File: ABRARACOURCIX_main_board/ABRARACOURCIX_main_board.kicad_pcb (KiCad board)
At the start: 2 copper layers, 140 x 140 mm, 78 parts, among them J1 Conn_01x05_Socket, J10 XT60PW-M, J11 Conn_01x02_Pin, J12 Conn_01x02_Pin, J2 Conn_01x06_Socket, J3 Conn_01x03_Socket, J4 Conn_01x03_Socket, J5 Conn_01x03_Socket, J6 Conn_01x03_Socket, J7 Conn_01x03_Socket, J8 XT60PW-M, J9 XT60PW-F, Q2 DSS20200L-7-PNP, Q3 IKD15N60R, Q4 NPN-DSS20201L-7, Q5 NTR4101PT1G, U1 STM32F429VITx, U2 BNO055, U3 Current_sens_ACS712ELCTR-20A-T, U4 AZ1117CH-3.3TRG1, U5 LMC6482AIMX/NOPB, U6 LMC6482AIMX/NOPB, Y1 ABS07-32.768KHZ-T

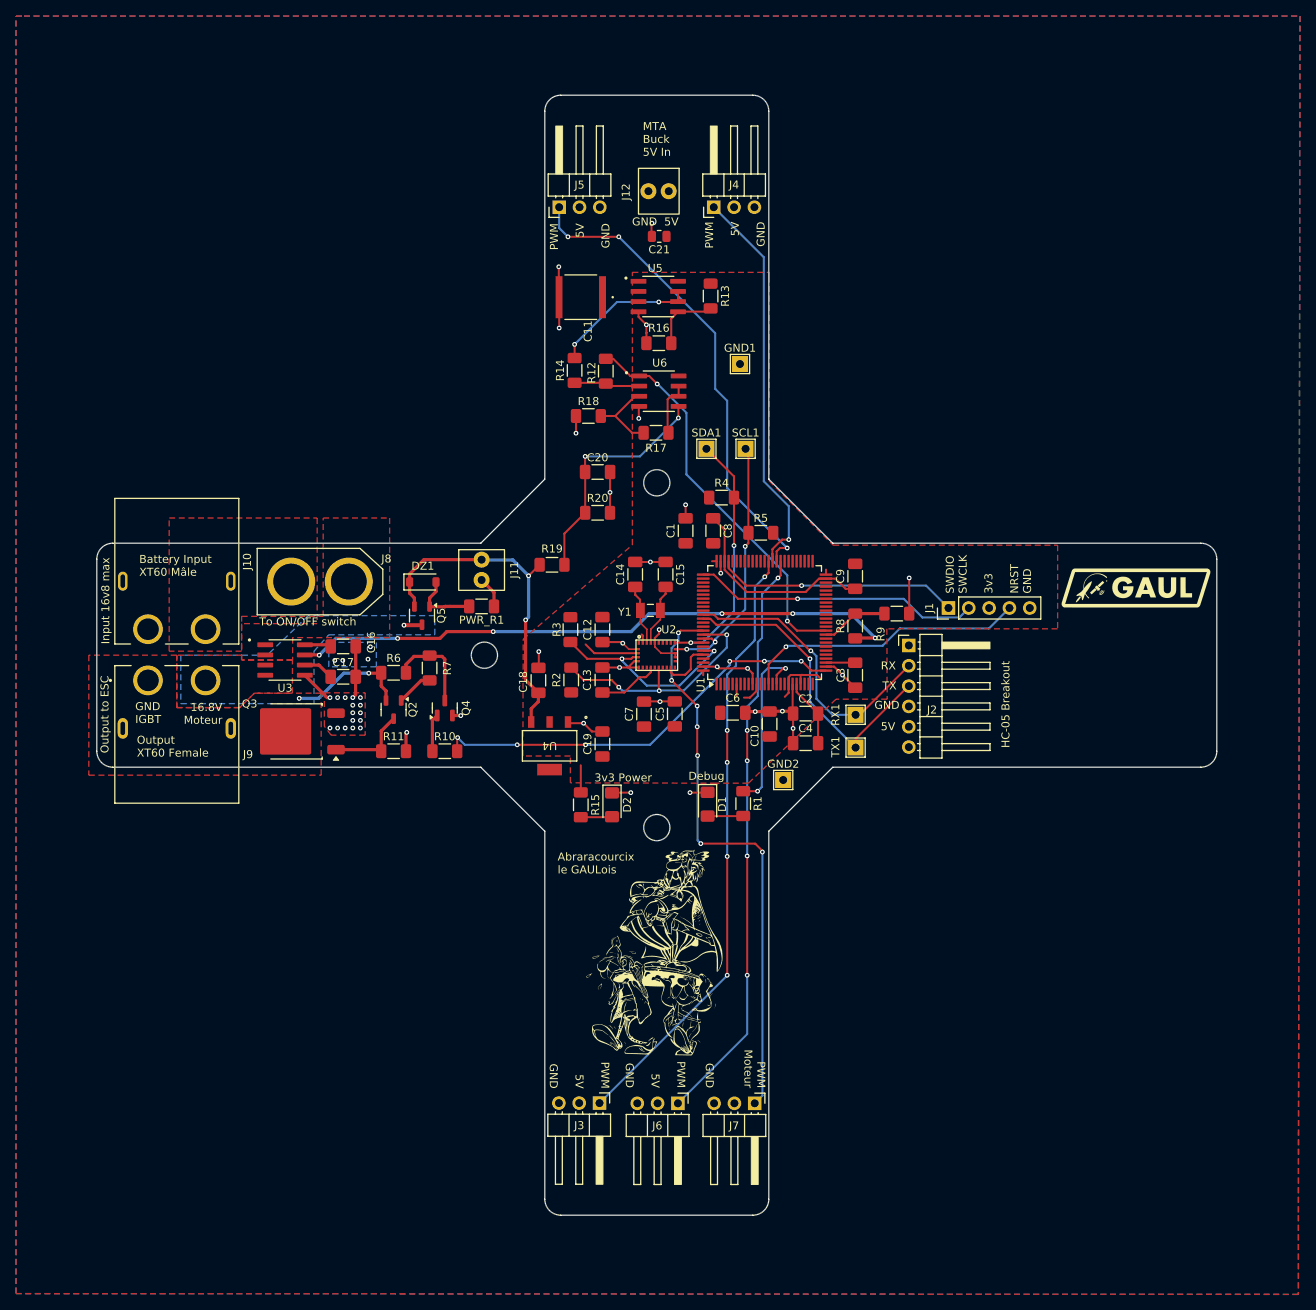
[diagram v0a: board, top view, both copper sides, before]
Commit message: Circuit+début PCB
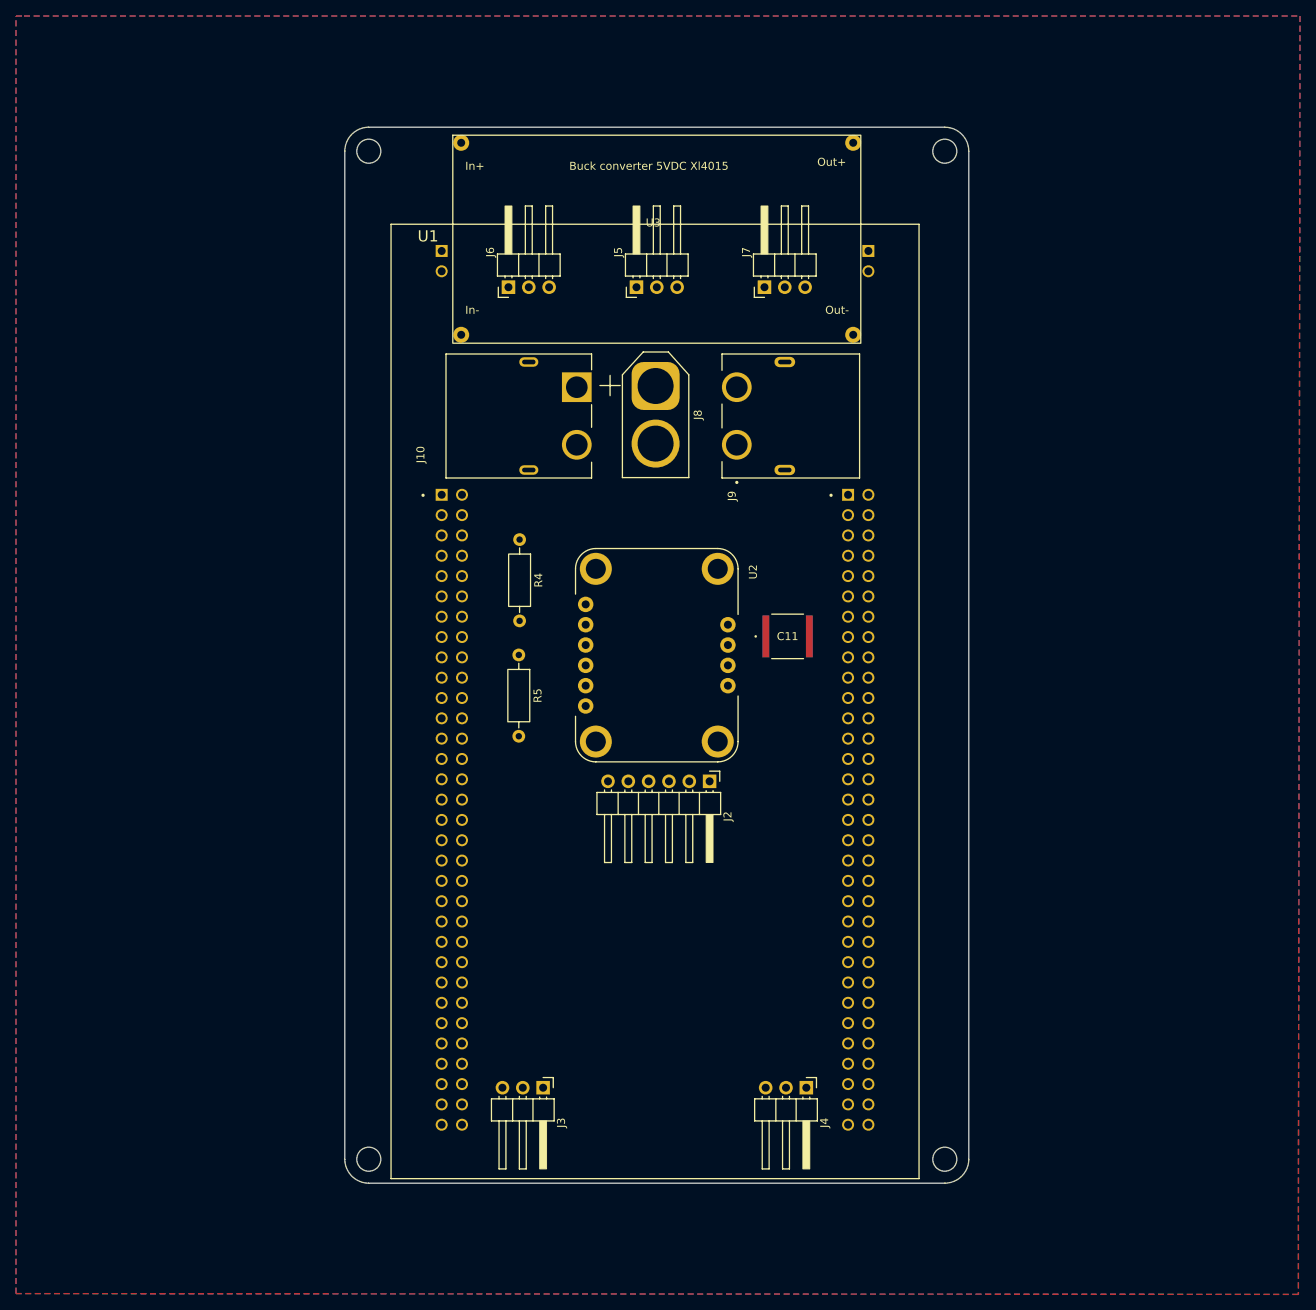
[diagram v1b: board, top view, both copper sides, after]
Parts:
- removed Abraracourcix_moyen: LOGO, Librairie_footprint:Abraracourcix_moyen
- removed C1, C2, C3, C5, C6: 100n, Capacitor_SMD:C_1206_3216Metric_Pad1.33x1.80mm_HandSolder
- removed C10, C20, C4: 1u, Capacitor_SMD:C_1206_3216Metric_Pad1.33x1.80mm_HandSolder
- removed C12: 100nF, Capacitor_SMD:C_1206_3216Metric_Pad1.33x1.80mm_HandSolder
- removed C13: 1uF, Capacitor_SMD:C_1206_3216Metric_Pad1.33x1.80mm_HandSolder
- removed C14, C15: 22pF, Capacitor_SMD:C_1206_3216Metric_Pad1.33x1.80mm_HandSolder
- removed C16: 0.1u, Capacitor_SMD:C_1206_3216Metric_Pad1.33x1.80mm_HandSolder
- removed C17: 1n, Capacitor_SMD:C_1206_3216Metric_Pad1.33x1.80mm_HandSolder
- removed C18: 10u, Capacitor_SMD:C_1206_3216Metric_Pad1.33x1.80mm_HandSolder
- removed C19: 22u, Capacitor_SMD:C_1206_3216Metric_Pad1.33x1.80mm_HandSolder
- removed C21: 22u, Resistor_SMD:R_0805_2012Metric
- removed C7: 4.7u, Capacitor_SMD:C_1206_3216Metric_Pad1.33x1.80mm_HandSolder
- removed C8, C9: 2.2u, Capacitor_SMD:C_1206_3216Metric_Pad1.33x1.80mm_HandSolder
- removed D1, D2: 599-0410-127F, Diode_SMD:D_1206_3216Metric_Pad1.42x1.75mm_HandSolder
- removed DZ1: SZMMSZ4679T1G, Diode_SMD:D_SOD-123
- removed G***1, G***2, G***3: LOGO, LOGO
- removed GND1, GND2, RX1, SCL1, SDA1, TX1: TestPoint, TestPoint:TestPoint_THTPad_2.0x2.0mm_Drill1.0mm
- removed J1: Conn_01x05_Socket, Connector_PinHeader_2.54mm:PinHeader_1x05_P2.54mm_Vertical
- removed J11, J12: Conn_01x02_Pin, Librairie_footprint:MTA_100_2pos
- removed PWR_R1: 100k, Resistor_SMD:R_1206_3216Metric_Pad1.30x1.75mm_HandSolder
- removed Q2: DSS20200L-7-PNP, Package_TO_SOT_SMD:SOT-23-3
- removed Q3: IKD15N60R, Package_TO_SOT_SMD:TO-252-2
- removed Q4: NPN-DSS20201L-7, Package_TO_SOT_SMD:SOT-23
- removed Q5: NTR4101PT1G, Package_TO_SOT_SMD:SOT-23-3
- removed R1, R15: 40, Resistor_SMD:R_1206_3216Metric_Pad1.30x1.75mm_HandSolder
- removed R10, R7: 1k5, Resistor_SMD:R_1206_3216Metric_Pad1.30x1.75mm_HandSolder
- removed R11, R13, R14, R17, R20, R6, R8: 10k, Resistor_SMD:R_1206_3216Metric_Pad1.30x1.75mm_HandSolder
- removed R12, R16, R18: 30k, Resistor_SMD:R_1206_3216Metric_Pad1.30x1.75mm_HandSolder
- removed R19: 40k, Resistor_SMD:R_1206_3216Metric_Pad1.30x1.75mm_HandSolder
- removed R2, R3: 10K, Resistor_SMD:R_1206_3216Metric_Pad1.30x1.75mm_HandSolder
- removed R9: 20k, Resistor_SMD:R_1206_3216Metric_Pad1.30x1.75mm_HandSolder
- removed U4: AZ1117CH-3.3TRG1, Librairie_footprint:AZ1117CH_3_3TRG1-L
- removed U5, U6: LMC6482AIMX/NOPB, Librairie_footprint:SOIC127P599X175-8N
- removed Y1: ABS07-32.768KHZ-T, Librairie_footprint:XTAL_ABS07-32.768KHZ-T
- added ?: , , F.Cu at (-36.0, 63.0)
- added ?: , , F.Cu at (-36.0, -62.1)
- added ?: , , F.Cu at (35.0, -63.8)
- added ?: , , F.Cu at (35.6, 63.0)
- R4, R5: footprint Resistor_SMD:R_1206_3216Metric_Pad1.30x1.75mm_HandSolder -> Resistor_THT:R_Axial_DIN0207_L6.3mm_D2.5mm_P10.16mm_Horizontal
- U1: value STM32F429VITx -> STM32F429I-DISC1; footprint Package_QFP:LQFP-100_14x14mm_P0.5mm -> Librairie_footprint:MODULE_STM32F429I-DISC1
- U2: value BNO055 -> BNO055_breakout; footprint Librairie_footprint:BNO055_LGA28R50P4X10_380X520X100 -> Librairie_footprint:MODULE_2472
- U3: value Current_sens_ACS712ELCTR-20A-T -> ~; footprint Librairie_footprint:Current_sens_SOIC127P600X175-8N -> Librairie_footprint:Buck_breakout_Xl4015
- moved J4 110.7 mm to (18.7, 54.1), turned to -90 degrees
- moved J6 103.7 mm to (-16.0, -46.0), turned to 90 degrees
- moved J7 102.1 mm to (16.0, -46.0), turned to 90 degrees
- moved J9 79.0 mm to (10.0, -33.5), turned to 90 degrees
- moved U3 70.2 mm to (0.00, -52.0)
- moved J10 55.6 mm to (-10.0, -33.5), turned to 90 degrees
- moved C11 49.7 mm to (16.4, -2.35), turned to 0 degrees
- moved J8 45.5 mm to (-0.15, -33.6), turned to -90 degrees
- moved R5 33.9 mm to (-17.2, -0.03), turned to -90 degrees
- moved J2 30.1 mm to (6.60, 15.8), turned to -90 degrees
- moved R4 25.8 mm to (-17.1, -14.4), turned to -90 degrees
- moved U1 16.9 mm to (-0.22, 5.78), turned to 0 degrees
- moved J5 15.8 mm to (0.00, -46.0)
- moved J3 7.31 mm to (-14.2, 54.1)
- turned U2 to -90 degrees
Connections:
- J2 pad 2: HC_RX -> +5V
- J2 pad 3: HC_TX -> GND
- J2 pad 4: GND -> HC_TX
- J2 pad 5: +5V -> HC_RX
- J9 pad 1: /Power/GND_IGBT -> GND
- J9 pad 2: /Power/16V_motor -> /Power/16V_post-switch
- U2 pad 1: (no net) -> +5V
- U2 pad 2: GND -> unconnected-(U2-3VO-Pad2)
- U2 pad 3: +3.3V -> GND
- U2 pad 4: BNO_BOOT -> SDA
- U2 pad 5: GND -> SCL
- U2 pad 6: GND -> BNO_Reset
- U2 pad 7: (no net) -> GND
- U2 pad 8: (no net) -> BNO_Int
- U2 pad 9: Net-(U2-CAP) -> unconnected-(U2-PS1-Pad9)
- U3 pad 1: /Power/16V_post-switch -> (no net)
- U3 pad 2: /Power/16V_post-switch -> (no net)
- U3 pad 3: /Power/16V_motor -> (no net)
- U3 pad 4: /Power/16V_motor -> (no net)
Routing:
- net GND: track 111.6 -> 0.00 mm, vias 43 -> 0
- net Net-(U3-VIOUT): track 77.4 -> 0.00 mm, vias 6 -> 0
- net PWM_Servo_4: track 76.5 -> 0.00 mm, vias 5 -> 0
- net PWM_Servo_1: track 73.1 -> 0.00 mm, vias 5 -> 0
- net PWM_Moteur: track 71.4 -> 0.00 mm, vias 7 -> 0
- net PWM_Servo_2: track 60.9 -> 0.00 mm, vias 3 -> 0
- net Motor_switch: track 53.4 -> 0.00 mm, vias 6 -> 0
- net PWM_Servo_3: track 49.5 -> 0.00 mm, vias 1 -> 0
- net VBAT_ADC: track 49.5 -> 0.00 mm, vias 2 -> 0
- net VBAT_sense: track 42.2 -> 0.00 mm, vias 2 -> 0
- net HC_TX: track 39.4 -> 0.00 mm, vias 1 -> 0
- net HC_RX: track 36.6 -> 0.00 mm, vias 1 -> 0
- net SYS_SWCLK: track 36.0 -> 0.00 mm, vias 1 -> 0
- net NRST: track 35.5 -> 0.00 mm, vias 1 -> 0
- net SCL: track 33.1 -> 0.00 mm, vias 3 -> 0
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- removed copper zone on F.Cu, net +3.3V
- removed copper zone on B.Cu, net +5V
- removed copper zone on B.Cu, net /Power/16V_motor
- removed copper zone on F.Cu, net /Power/16V_motor
- removed copper zone on F.Cu, net /Power/16V_post-switch
- removed copper zone on F.Cu, net /Power/16V_pre-switch
- removed copper zone on F.Cu, net /Power/GND_IGBT
- removed copper zone on F.Cu, net GND
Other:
- board size 140 x 140 mm -> 78 x 132 mm
- board text removed: "16.8V"
- board text removed: "16.8V Moteur"
- board text removed: "3v3 Power"
- board text removed: "5V"
- board text removed: "5V GND"
- board text removed: "Abraracourcix le GAULois"
- board text removed: "Battery Input"
- board text removed: "Battery Input XT60 Mâle"
- board text removed: "Debug"
- board text removed: "GND"
- board text removed: "GND 5V"
- board text removed: "GND IGBT"
- board text removed: "HC-05 Breakout"
- board text removed: "Input 16v8 max"
- board text removed: "MTA Buck 5V In"
- board text removed: "Output XT60 Female"
- board text removed: "Output to ESC"
- board text removed: "PWM 5V GND"
- board text removed: "PWM Moteur GND"
- board text removed: "Projet ABRARACOURCIX V1 GAULxDesign IV 2025 Nathan Armishaw Etienne Bernier Marc-André Tremblay Rémi Plante Félix Dion"
- board text removed: "Projet ABRARACOURCIX: Asservissement en Boucles et Régulation Avancée RApide pour le Contrôle d'Objet Unirotorisé Réactifs avec Capteur Inertiel eXpérimental"
- board text removed: "RX"
- board text removed: "SCL"
- board text removed: "SDA"
- board text removed: "SWDIO SWCLK 3v3 NRST GND"
- board text removed: "TX"
- board text removed: "To ON/OFF switch"
